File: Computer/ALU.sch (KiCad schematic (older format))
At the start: 24 parts, among them J1 Conn_01x08, J2 Conn_01x01, J3 Conn_01x04, J4 Conn_01x01, J5 Conn_01x01, J6 Conn_01x01, U1 74LS253, U10 74LS08, U11 74LS283, U12 74LS283, U13 74LS257, U14 74LS257, U15 74LS257, U16 74LS257, U17 74LS574, U18 74LS574, U2 74LS253, U3 74LS253, U4 74LS253, U5 74LS253, U6 74LS253, U7 74LS253, U8 74LS253, U9 74LS04

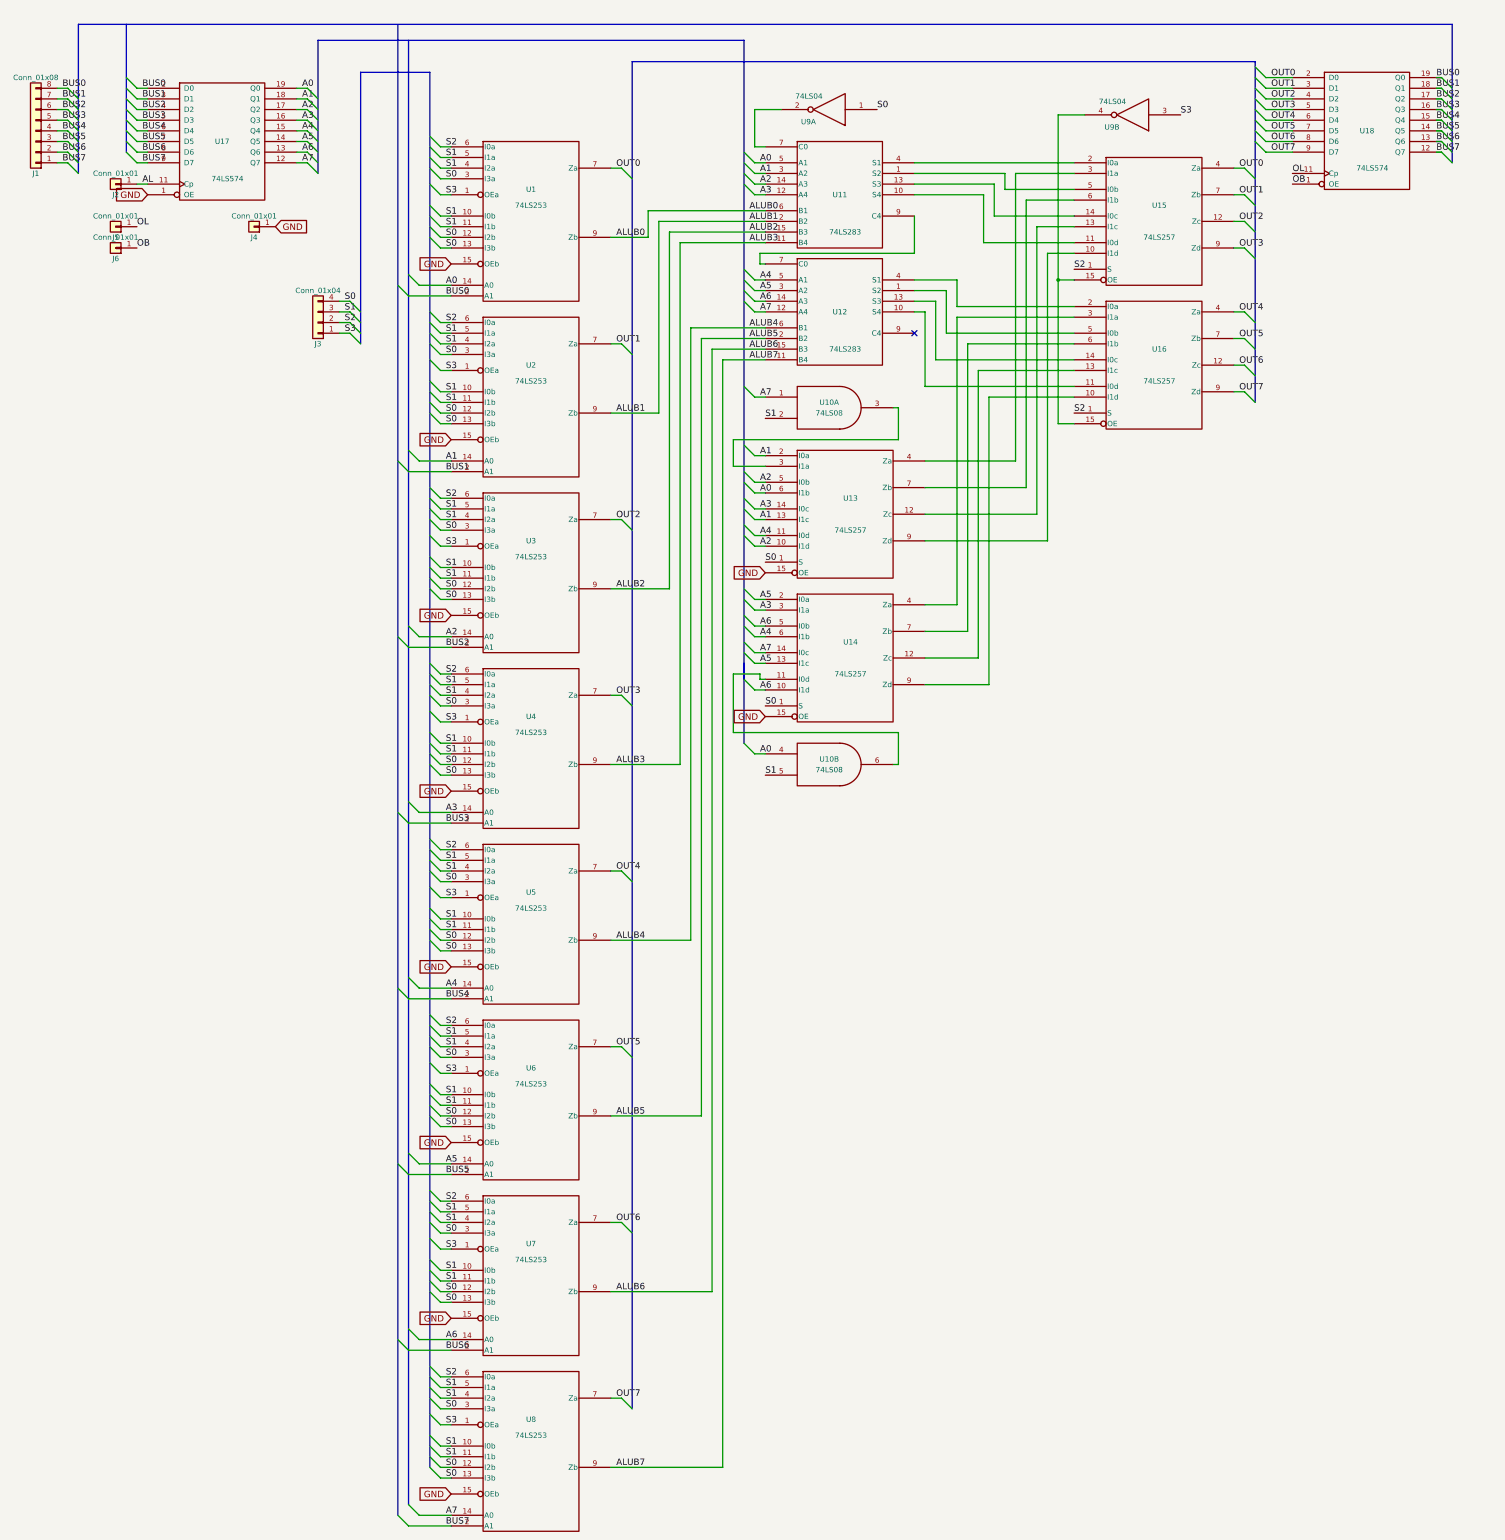
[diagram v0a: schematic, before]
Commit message: updates
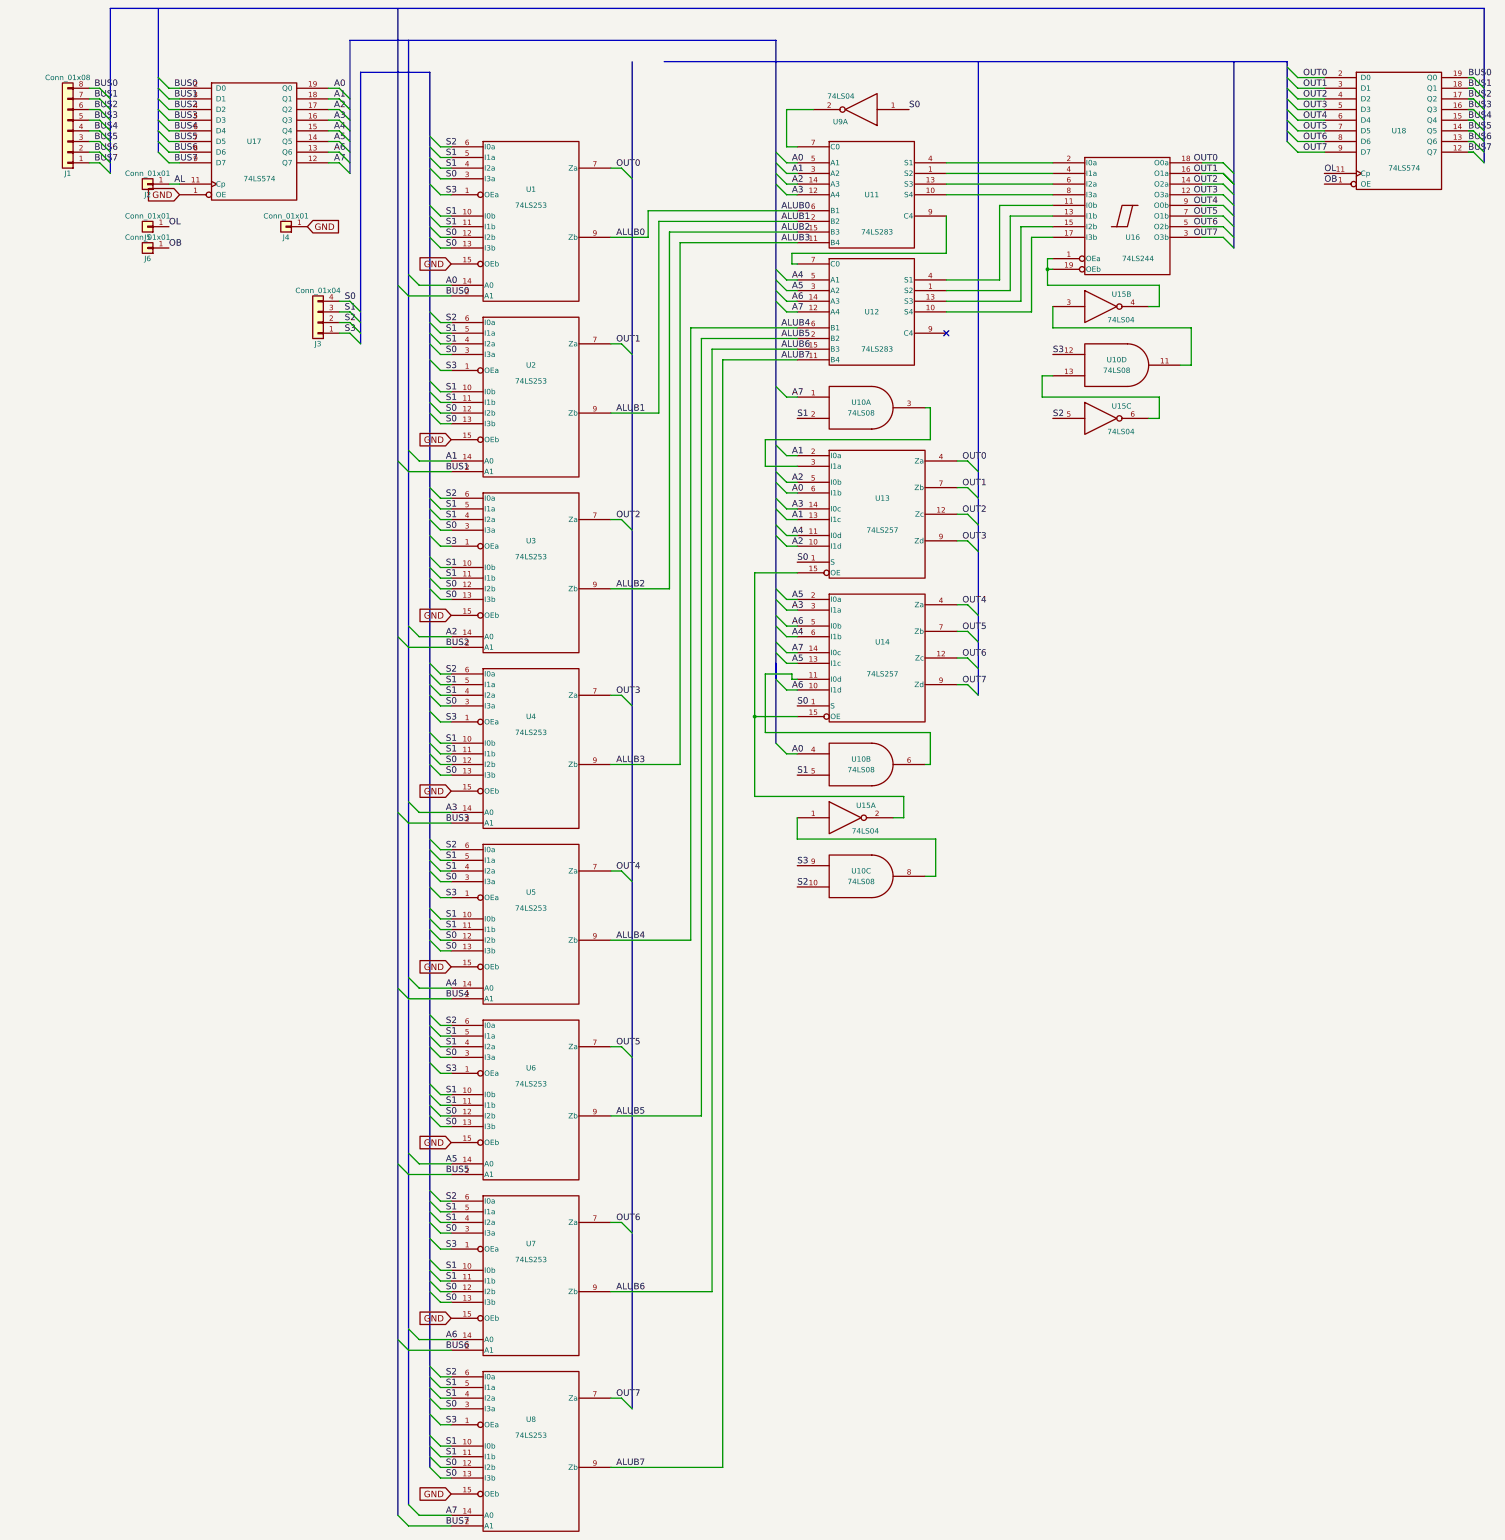
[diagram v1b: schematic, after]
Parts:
- removed U15, U16: 74LS257, Housings_DIP:DIP-16_W7.62mm, symbol 74LS257
- removed unit 2 of U9
- added unit 3 of U10
- added unit 4 of U10
- added U15: 74LS04, Housings_DIP:DIP-14_W7.62mm, symbol 74LS04
- added U16: 74LS244, Housings_DIP:DIP-14_W7.62mm, symbol 74LS244
- J1: footprint Pin_Headers:Pin_Header_Angled_1x08_Pitch2.00mm -> Pin_Headers:Pin_Header_Straight_1x08_Pitch1.00mm
- J2: footprint Pin_Headers:Pin_Header_Angled_1x01_Pitch1.00mm -> Pin_Headers:Pin_Header_Straight_1x01_Pitch2.00mm
- J3: footprint Pin_Headers:Pin_Header_Angled_1x04_Pitch2.00mm -> Pin_Headers:Pin_Header_Straight_1x04_Pitch1.00mm
- J4, J5, J6: footprint Pin_Headers:Pin_Header_Angled_1x01_Pitch1.00mm -> Pin_Headers:Pin_Header_Straight_1x01_Pitch1.00mm
- U17, U18: footprint (none) -> Housings_DIP:DIP-14_W7.62mm
- U9: footprint Housings_DIP:DIP-14_W7.62mm -> Housings_DIP:DIP-16_W7.62mm
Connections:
- net GND: now also U10.7 (GND), U10.7 (GND), U15.7 (GND), U15.7 (GND), U15.7 (GND), U16.10 (GND); no longer U13.15 (OE), U14.15 (OE)
- net OUT0: now also U13.4 (Za), U16.18 (O0a)
- net OUT1: now also U13.7 (Zb), U16.16 (O1a)
- net OUT2: now also U13.12 (Zc), U16.14 (O2a)
- net OUT3: now also U13.9 (Zd), U16.12 (O3a)
- net OUT4: now also U14.4 (Za), U16.9 (O0b)
- net OUT5: now also U14.7 (Zb), U16.7 (O1b)
- net OUT6: now also U14.12 (Zc), U16.5 (O2b)
- net OUT7: now also U14.9 (Zd), U16.3 (O3b)
- net S2: now also U10.10, U15.5
- net S3: now also U10.12, U10.9
- net VCC: now also U10.14 (VCC), U10.14 (VCC), U15.14 (VCC), U15.14 (VCC), U15.14 (VCC), U16.20 (VCC)
- net at U11.1 (S2): now also U16.4 (I1a)
- net at U11.10 (S4): now also U16.8 (I3a)
- net at U11.13 (S3): now also U16.6 (I2a)
- net at U11.4 (S1): now also U16.2 (I0a)
- net at U12.1 (S2): now also U16.13 (I1b)
- net at U12.10 (S4): now also U16.17 (I3b)
- net at U12.13 (S3): now also U16.15 (I2b)
- net at U12.4 (S1): now also U16.11 (I0b)
- new net: U13.15 (OE), U14.15 (OE), U15.2
- new net: U15.4, U16.1 (OEa), U16.19 (OEb)
- new net: U10.8, U15.1
- new net: U10.13, U15.6
- new net: U10.11, U15.3
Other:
- moved on the sheet: J1, J2, J4, J5, J6, U10A, U10B, U11, U12, U13, U14, U17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
